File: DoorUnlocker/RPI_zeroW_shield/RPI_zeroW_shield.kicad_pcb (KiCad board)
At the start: 2 copper layers, 25.9 x 27.4 mm, 11 parts, among them J3 ServoConn, J4 ReedConn, J5 ButtonConn, K1 SANYOU_SRD_Form_C, Q1 BC547

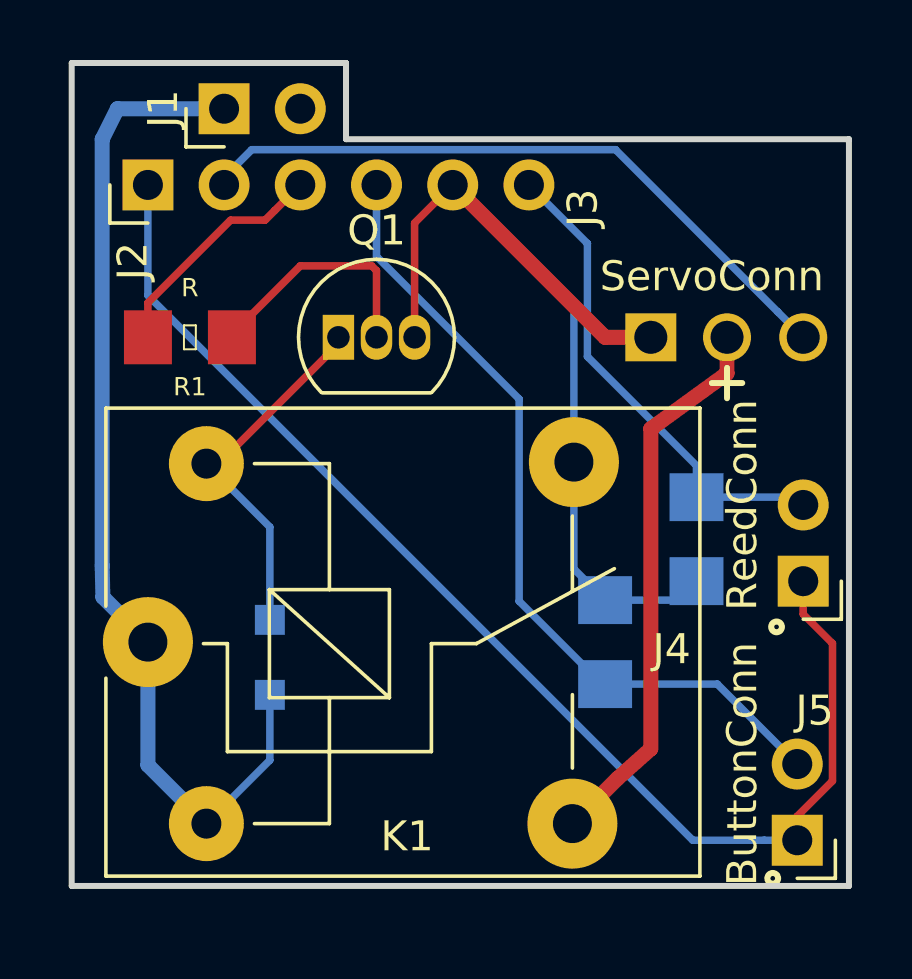
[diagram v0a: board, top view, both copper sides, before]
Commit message: pcb updates
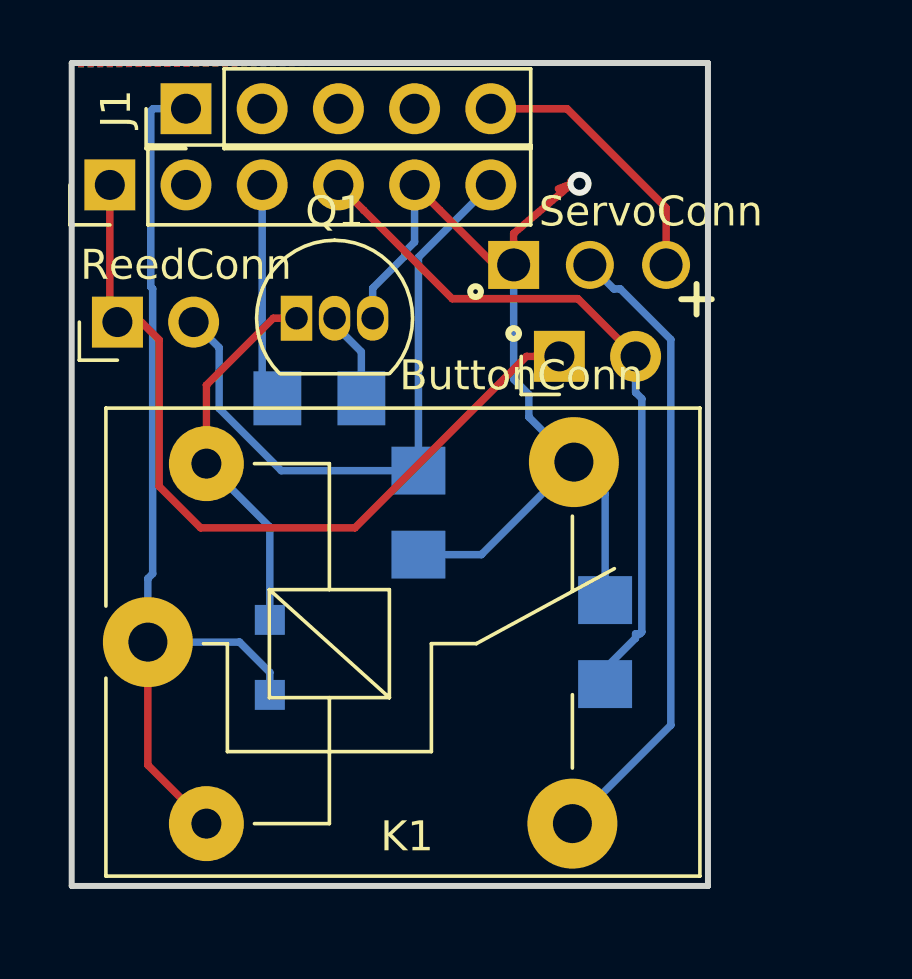
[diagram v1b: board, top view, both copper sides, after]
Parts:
- J1: value (none) -> Conn_01x05_Male; footprint CustomFP:PinHeader_1x02_P2.54mm_Horizontal -> Connector_PinHeader_2.54mm:PinHeader_1x05_P2.54mm_Vertical
- J2: value (none) -> Conn_01x06_Male; footprint CustomFP:PinHeader_1x06_P2.54mm_Horizontal -> Connector_PinHeader_2.54mm:PinHeader_1x06_P2.54mm_Vertical
- R1: moved to B.Cu
- moved J4 24.4 mm to (118.4, 63.0), turned to 90 degrees
- moved J5 18.0 mm to (133.1, 64.1), turned to 90 degrees
- moved R2 9.31 mm to (128.4, 69.3)
- moved J3 5.17 mm to (131.6, 61.1)
- moved R1 4.77 mm to (125.1, 65.5)
- moved Q1 1.53 mm to (124.3, 62.9)
- moved J1 1.27 mm to (120.7, 55.9)
- moved J2 1.27 mm to (118.1, 58.4)
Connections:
- J2 pad 2: /ServoPWM_P2 -> (no net)
- J3 pad 3: /ServoPWM_P2 -> /ServoPWM_P18
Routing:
- net /ServoPWM_P2: track 22.5 -> 0.00 mm
- net /3V3_IN: track 42.4 -> 27.5 mm
- net /ServoPWM_P18: track 0.00 -> 9.11 mm
- net Net-(Q1-Pad2): track 8.15 -> 3.04 mm
- net /Reed_P17: track 16.4 -> 21.3 mm
- net /Button_P4: track 27.4 -> 23.9 mm
- net /5v_IN: track 34.1 -> 31.1 mm
- net Net-(J3-Pad2): track 18.6 -> 21.2 mm
- net GND: track 33.6 -> 33.0 mm, vias 0 -> 1
- net /Relay_P3: track 7.86 -> 7.32 mm
- added copper zone on B.Cu, net GND
- added copper zone on F.Cu, net GND
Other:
- board size 25.9 x 27.4 mm -> 21.2 x 27.4 mm
